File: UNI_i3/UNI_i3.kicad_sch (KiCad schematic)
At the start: 160 parts, among them J1 Conn_01x19_Pin, J2 Conn_01x19_Pin, SW1 MX_SW_solder, SW10 MX_SW_solder, SW11 MX_SW_solder, SW12 MX_SW_solder, SW13 MX_SW_solder, SW14 MX_SW_solder, SW15 MX_SW_solder, SW16 MX_SW_solder, SW17 MX_SW_solder, SW18 MX_SW_solder, SW19 MX_SW_solder, SW2 MX_SW_solder, SW20 MX_SW_solder, SW21 MX_SW_solder, SW22 MX_SW_solder, SW23 MX_SW_solder, SW24 MX_SW_solder, SW25 MX_SW_solder, SW26 MX_SW_solder, SW27 MX_SW_solder, SW28 MX_SW_solder, SW29 MX_SW_solder, SW3 MX_SW_solder, SW30 MX_SW_solder, SW31 MX_SW_solder, SW32 RotaryEncoder_Switch, SW33 MX_SW_solder, SW34 MX_SW_solder, SW35 MX_SW_solder, SW36 MX_SW_solder, SW37 MX_SW_solder, SW38 MX_SW_solder, SW39 MX_SW_solder, SW4 MX_SW_solder, SW40 MX_SW_solder, SW41 MX_SW_solder, SW42 MX_SW_solder, SW43 MX_SW_solder, SW44 MX_SW_solder, SW45 MX_SW_solder, SW46 MX_SW_solder, SW47 MX_SW_solder, SW48 RotaryEncoder_Switch, SW49 MX_SW_solder, SW5 MX_SW_solder, SW50 MX_SW_solder, SW51 MX_SW_solder, SW52 MX_SW_solder, SW53 MX_SW_solder, SW54 MX_SW_solder, SW55 MX_SW_solder, SW56 MX_SW_solder, SW57 MX_SW_solder, SW58 MX_SW_solder, SW59 MX_SW_solder, SW6 MX_SW_solder, SW60 MX_SW_solder, SW61 MX_SW_solder, SW62 MX_SW_solder, SW63 MX_SW_solder, SW64 MX_SW_solder, SW65 MX_SW_solder, SW66 MX_SW_solder, SW67 MX_SW_solder, SW68 MX_SW_solder, SW69 MX_SW_solder, SW7 MX_SW_solder, SW70 MX_SW_solder, SW71 MX_SW_solder, SW72 MX_SW_solder, SW73 MX_SW_solder, SW74 MX_SW_solder, SW75 MX_SW_solder, SW76 SW_Push_45deg, SW8 MX_SW_solder, SW9 MX_SW_solder, U1 Bonsai-C4-extended

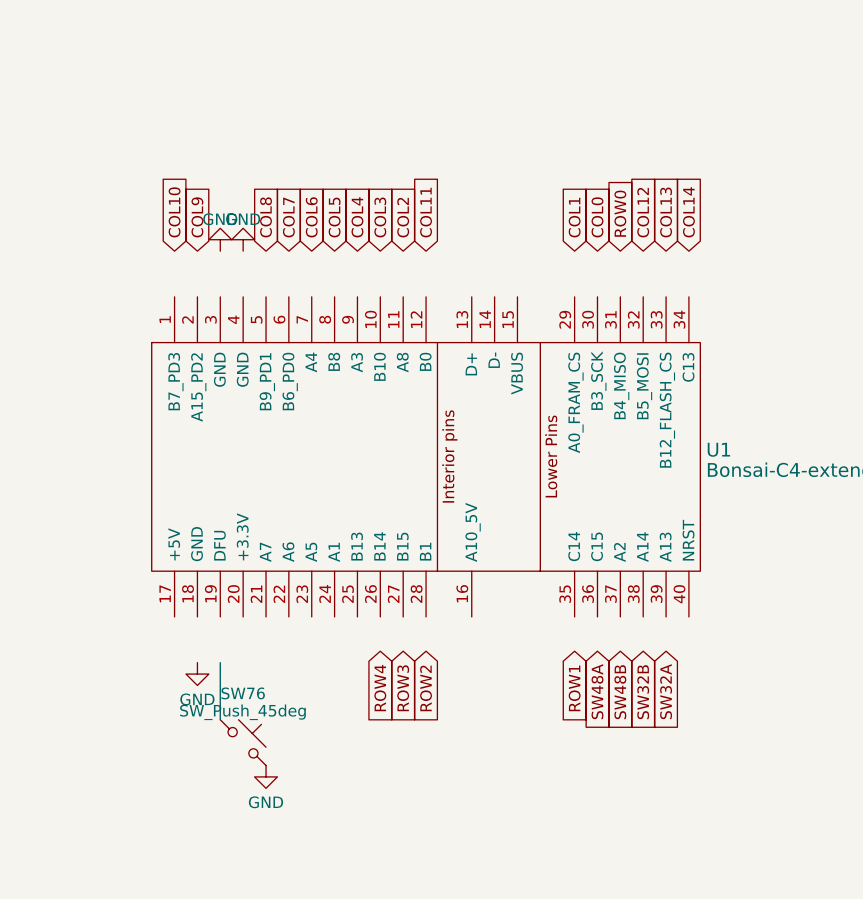
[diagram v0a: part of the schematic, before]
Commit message: uni_i3
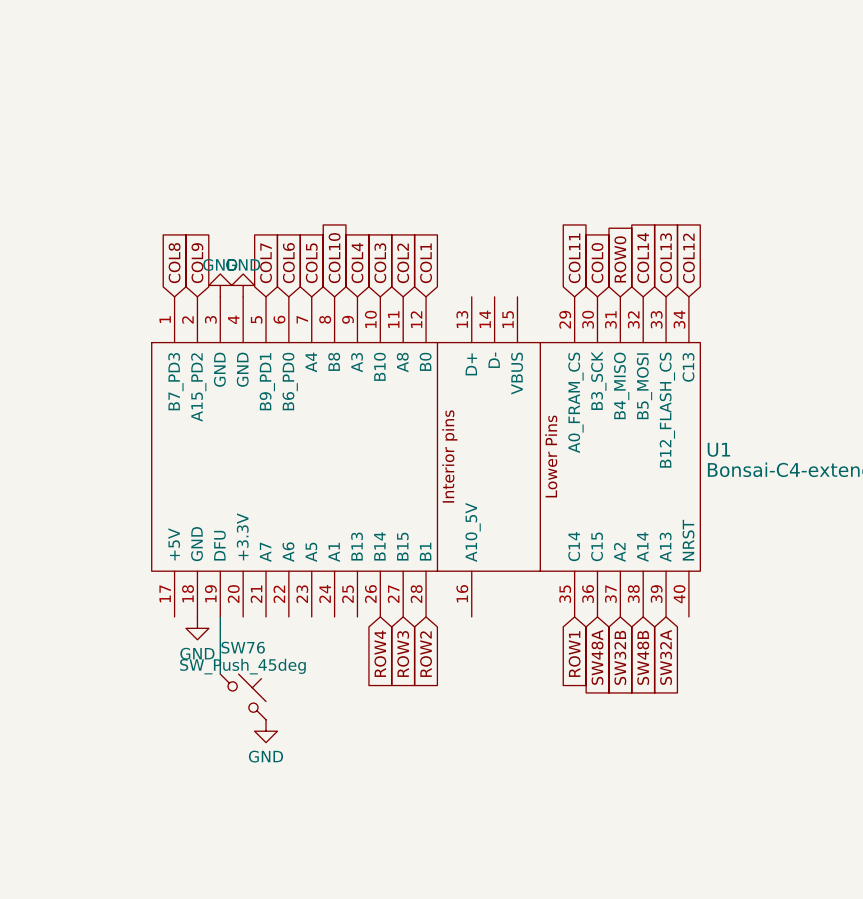
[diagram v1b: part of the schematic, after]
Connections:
- net COL0: now also U1.30 (B3_SCK)
- net COL1: now also U1.12 (B0)
- net COL10: now also U1.8 (B8)
- net COL11: now also U1.29 (A0_FRAM_CS)
- net COL12: now also U1.34 (C13)
- net COL13: now also U1.33 (B12_FLASH_CS)
- net COL14: now also U1.32 (B5_MOSI)
- net COL2: now also U1.11 (A8)
- net COL3: now also U1.10 (B10)
- net COL4: now also U1.9 (A3)
- net COL5: now also U1.7 (A4)
- net COL6: now also U1.6 (B6_PD0)
- net COL7: now also U1.5 (B9_PD1)
- net COL8: now also U1.1 (B7_PD3)
- net COL9: now also U1.2 (A15_PD2)
- net GND: now also U1.18 (GND), U1.3 (GND), U1.4 (GND)
- net ROW0: now also U1.31 (B4_MISO)
- net ROW1: now also U1.35 (C14)
- net ROW2: now also U1.28 (B1)
- net ROW3: now also U1.27 (B15)
- net ROW4: now also U1.26 (B14)
- net SW32A: now also U1.39 (A13)
- net SW32B: now also U1.37 (A2)
- net SW48A: now also U1.36 (C15)
- net SW48B: now also U1.38 (A14)
- net at SW76.1: now also U1.19 (DFU)
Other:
- moved on the sheet: SW76
